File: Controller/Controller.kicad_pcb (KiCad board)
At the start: 2 copper layers, 14 x 9 mm, 10 parts, among them SW1 SW_DPST_x2

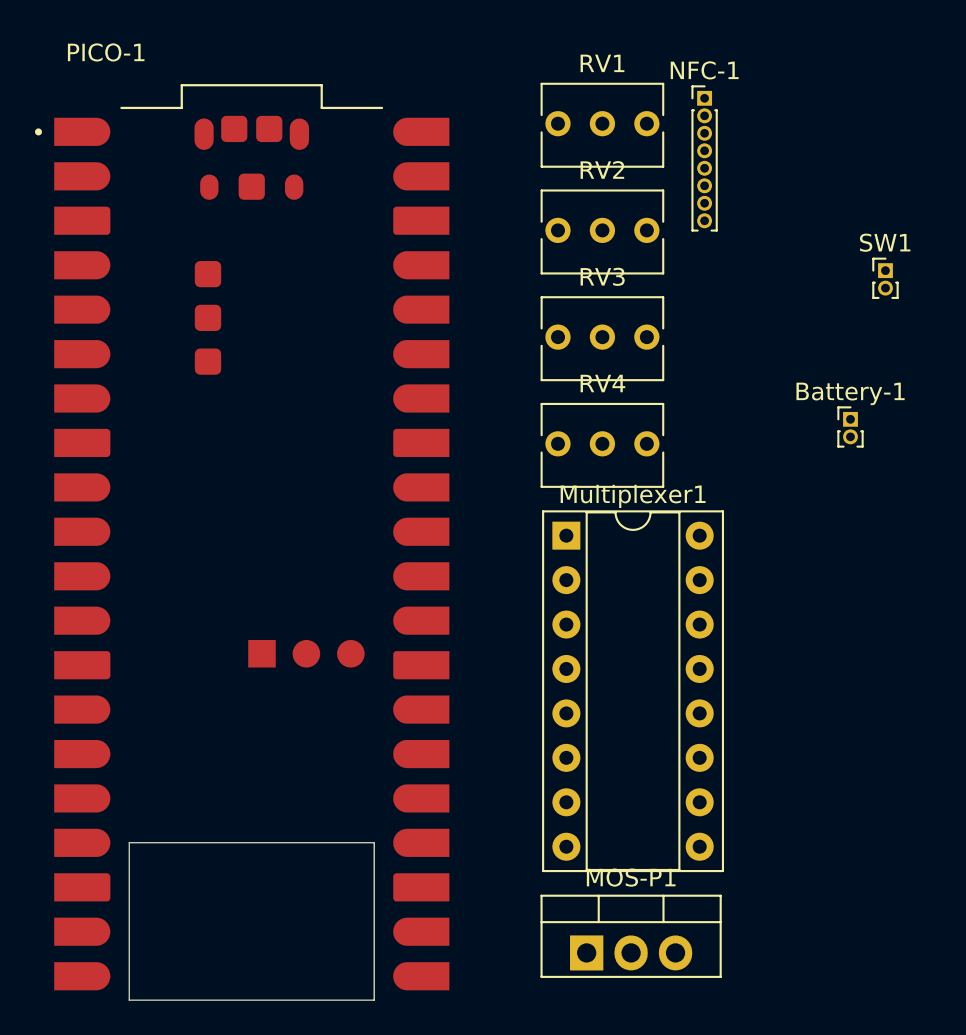
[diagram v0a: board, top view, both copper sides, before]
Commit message: Add sections
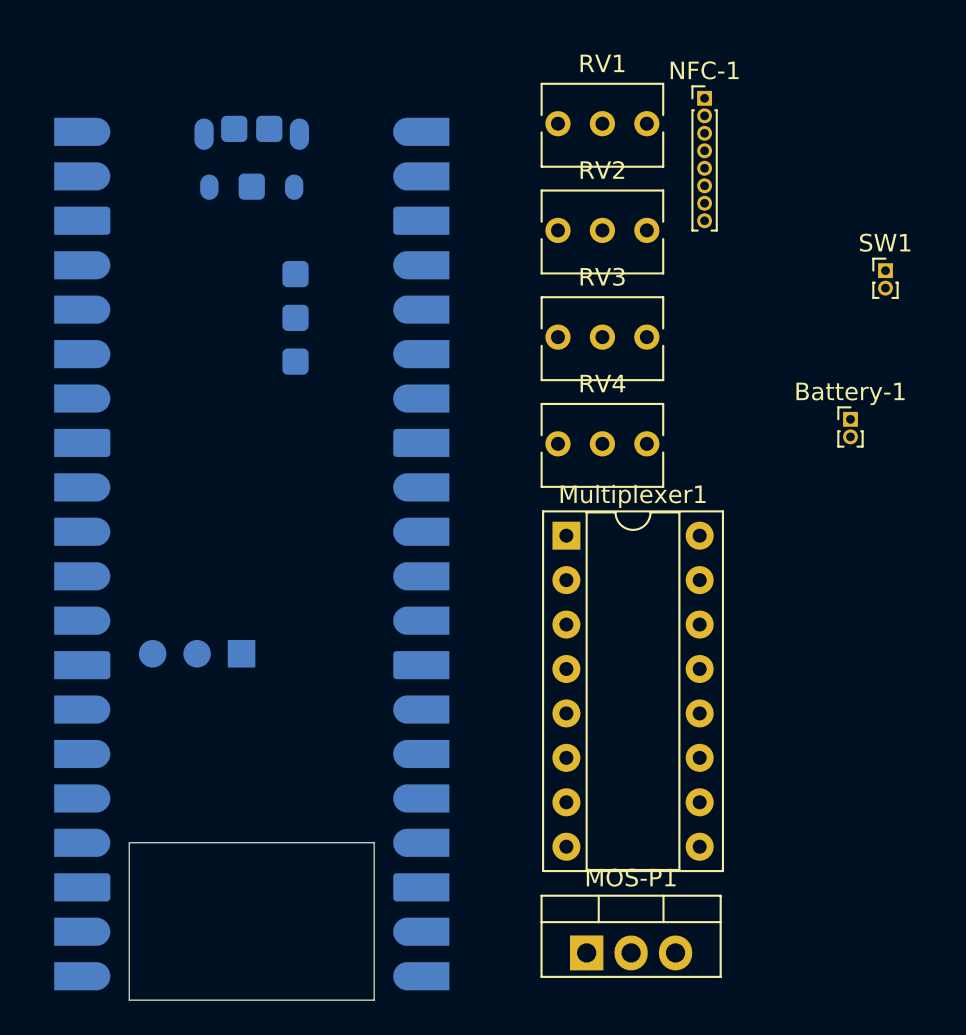
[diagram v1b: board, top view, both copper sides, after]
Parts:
- PICO-1: moved to B.Cu
- turned PICO-1 to 180 degrees
